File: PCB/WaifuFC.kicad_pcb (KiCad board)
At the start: 2 copper layers, 40.2 x 38.1 mm, 58 parts, among them J1 SBUS, J2 USB_C_Receptacle_USB2.0, J3 PPM, J4 OUT, J5 Conn_01x02, J6 Conn_01x02, J7 Conn_01x04, Q1 1P, SW1 SW_Push, U1 STM32F103C8Tx, U2 MPU-6050, U3 MP1584, U4 AZ1117-3.3, Y1 8MHz

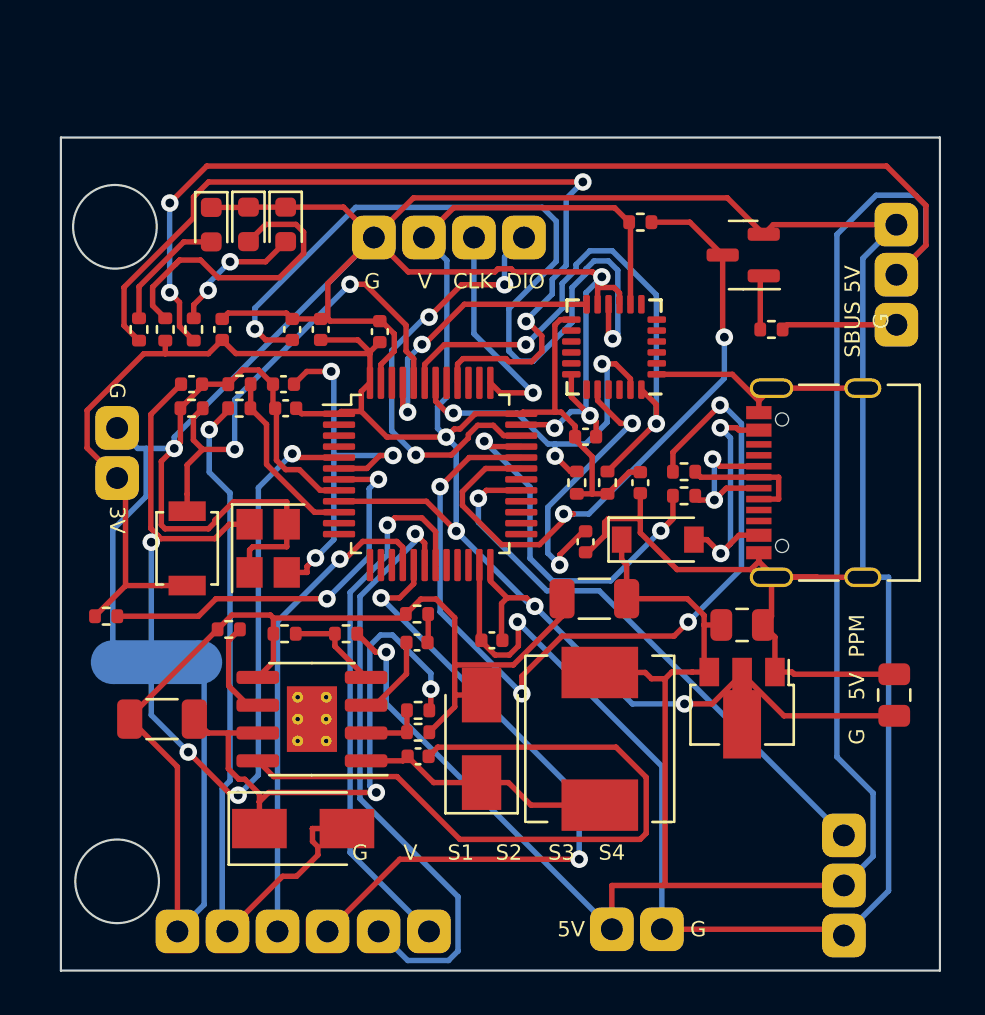
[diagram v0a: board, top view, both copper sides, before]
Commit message: v3
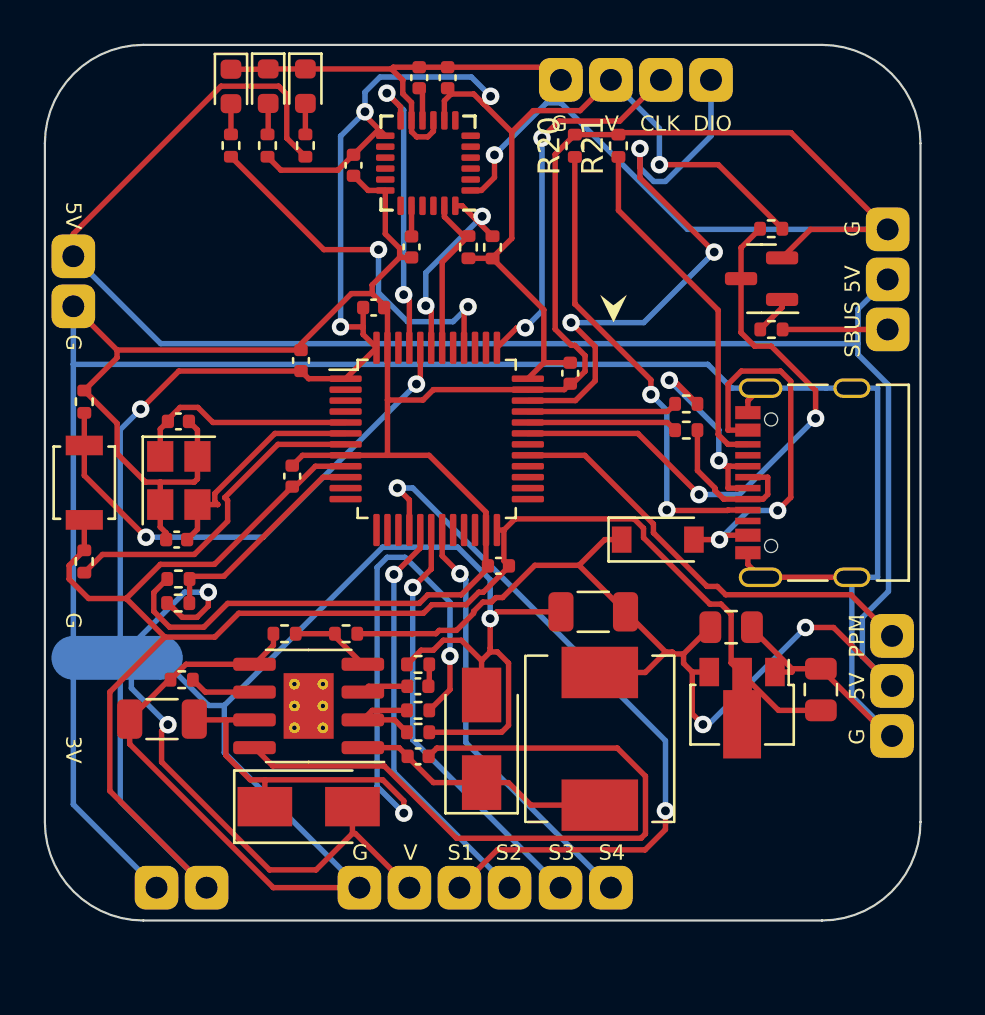
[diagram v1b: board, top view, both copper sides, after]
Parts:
- added G***: LOGO, SFA_LOGO:Arrow, F.Cu at (145.7, 89.3)
- added R20: R, Resistor_SMD:R_0402_1005Metric, F.Cu at (143.9, 81.8)
- added R21: R, Resistor_SMD:R_0402_1005Metric, F.Cu at (145.9, 81.8)
- moved J5 39.1 mm to (121.0, 89.1), turned to 0 degrees
- moved J6 21.1 mm to (124.8, 115.7), turned to -90 degrees
- moved C11 15.6 mm to (136.4, 86.4)
- moved C9 12.9 mm to (136.8, 78.7)
- moved C8 12.9 mm to (138.1, 78.7)
- moved R3 12.0 mm to (140.2, 86.5)
- moved U2 12.0 mm to (137.2, 82.6)
- moved R4 11.8 mm to (139.1, 86.4)
- moved C2 11.3 mm to (134.7, 89.2)
- moved J7 11.2 mm to (143.3, 78.8)
- moved R17 9.83 mm to (131.6, 81.8)
- moved R16 9.61 mm to (129.9, 81.8)
- moved R15 9.39 mm to (128.2, 81.8)
- moved J3 9.38 mm to (158.4, 107.9)
- moved R18 9.33 mm to (125.8, 102.7)
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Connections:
- J2 pad A5: unconnected-(J2-PadA5) -> Net-(J2-CC1)
- J2 pad B5: unconnected-(J2-PadB5) -> Net-(J2-CC2)
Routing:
- net +3V3: track 124.5 -> 176.8 mm, vias 4 -> 5
- net /REGOUT: track 38.8 -> 1.53 mm, vias 2 -> 0
- net /HSE_IN: track 44.8 -> 10.5 mm, vias 4 -> 0
- net /USB_DN: track 40.6 -> 6.87 mm, vias 4 -> 0
- net GND: track 239.7 -> 265.5 mm, vias 5 -> 1
- net +5V: track 142.1 -> 116.6 mm, vias 3 -> 2
- net /LED_STATUS: track 40.5 -> 17.3 mm
- net Net-(J2-CC1): track 0.00 -> 21.6 mm, vias 0 -> 2
- net /IMU_SDA: track 26.1 -> 9.76 mm
- net GNDPWR: track 57.7 -> 74.0 mm, vias 0 -> 1
- net Net-(J2-CC2): track 0.00 -> 16.1 mm
- net /USB_DP: track 20.3 -> 6.87 mm, vias 2 -> 0
- net Net-(D4-A): track 14.1 -> 1.43 mm
- net /VIN: track 26.0 -> 38.2 mm
- net /TIM3_S2: track 31.2 -> 19.0 mm, vias 2 -> 1
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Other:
- board size 40.2 x 38.1 mm -> 40 x 40 mm
